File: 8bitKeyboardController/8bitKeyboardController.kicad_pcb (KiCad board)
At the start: 2 copper layers, 93.5 x 55 mm, 14 parts

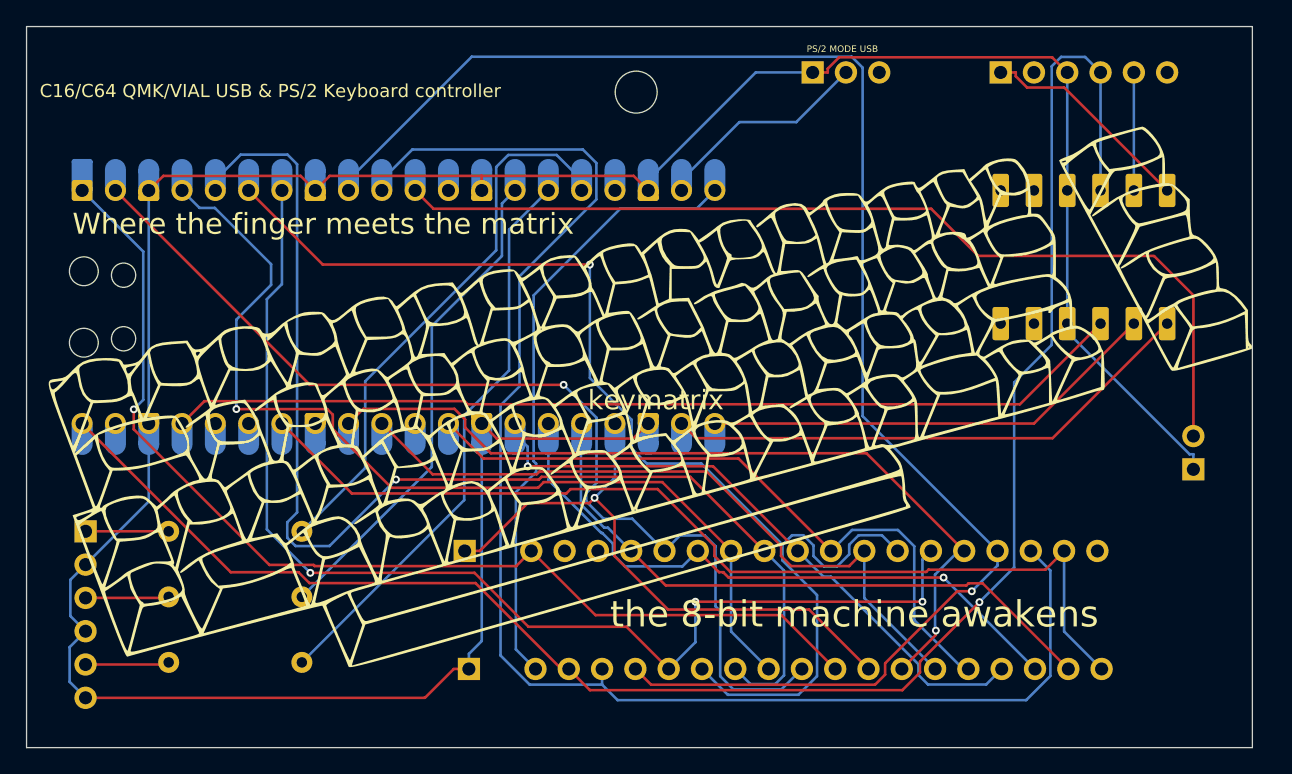
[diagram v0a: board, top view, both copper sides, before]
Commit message: visual update
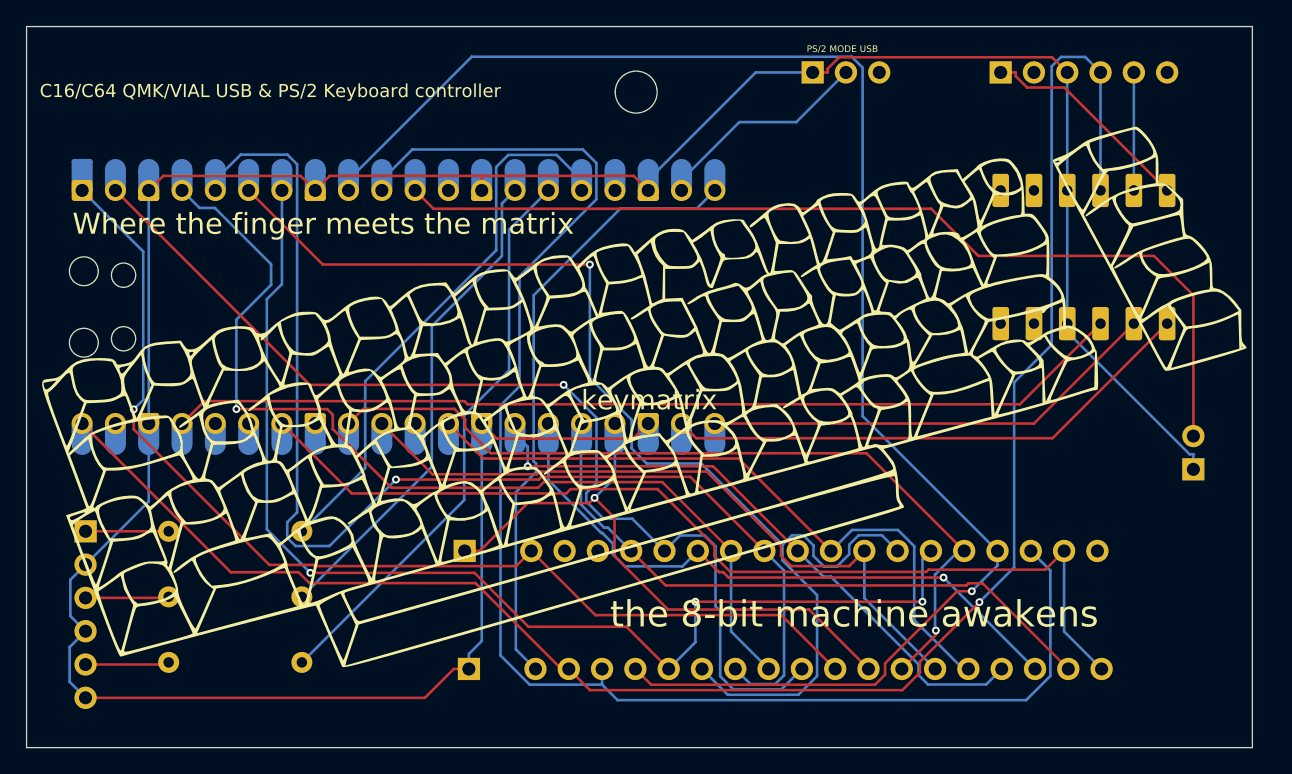
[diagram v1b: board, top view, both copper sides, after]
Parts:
- moved keymatrix 0.50 mm to (151.0, 102.5)
